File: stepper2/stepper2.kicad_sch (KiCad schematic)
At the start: 20 parts, among them J1 DB25_Socket, J2 Conn_02x10_Odd_Even, J3 DB25_Pins, J4 Conn_02x10_Odd_Even, J5 Blue Pill, J6 IPS 240*240, SW2 SW_Push, SW3 SW_Push, SW4 SW_SPDT, SW5 SW_Push_SPDT

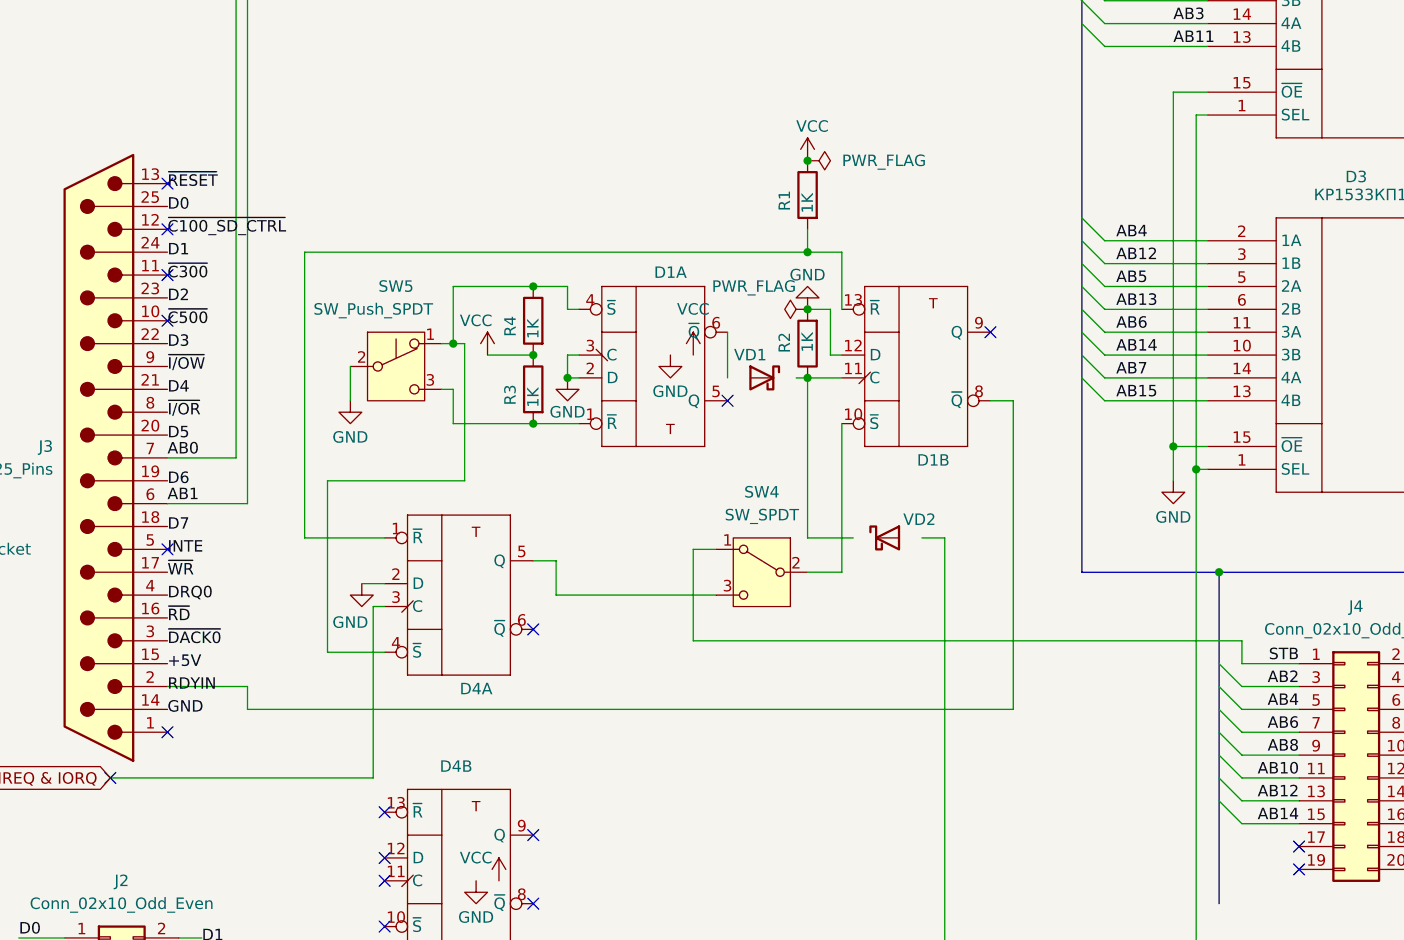
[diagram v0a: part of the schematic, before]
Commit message: Fix stepper
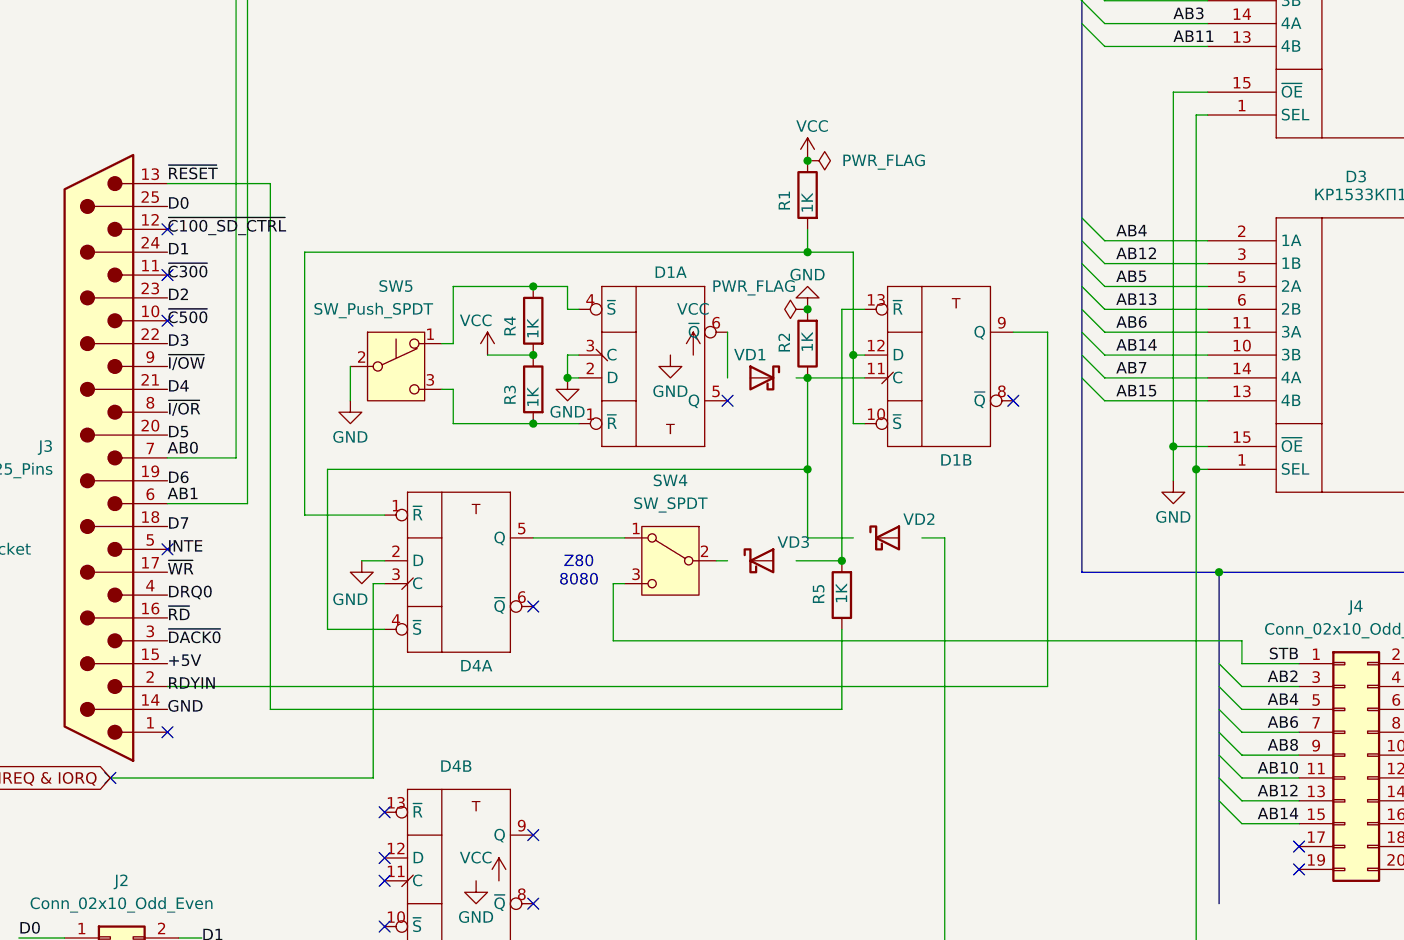
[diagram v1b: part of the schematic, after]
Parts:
- added unit 2 of D4
- added R5: 1K, Resistor_THT:R_Axial_DIN0207_L6.3mm_D2.5mm_P5.08mm_Vertical, symbol Device:R
- added VD3: 1N4148, Diode_THT:D_DO-34_SOD68_P2.54mm_Vertical_AnodeUp, symbol Diode:BAT43
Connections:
- net GND: now also D4.7 (GND); no longer D1.12 (D)
- net RDYIN: now also D1.9 (Q); no longer D1.8 (~{Q})
- net STB: now also SW4.3 (C); no longer SW4.1 (A)
- net VCC: now also D4.14 (VCC)
- net ~{RESET}: now also R5.1
- net at SW4.2 (B): no longer D1.10 (~{S})
- net at D4.5 (Q): now also SW4.1 (A); no longer SW4.3 (C)
- net at D4.1 (~{R}), R1.2: now also D1.10 (~{S}), D1.12 (D); no longer D1.13 (~{R})
- net at D1.4 (~{S}), R4.1, SW5.1 (A): no longer D4.4 (~{S})
- net at D1.11 (C), R2.1: now also D4.4 (~{S})
- new net: D1.13 (~{R}), R5.2
- no-connect marks 56 -> 55
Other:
- note added: "Z80 8080"
- moved on the sheet: D1B, D4A, SW4
